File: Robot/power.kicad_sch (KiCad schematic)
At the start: 34 parts, among them J16 Battery, J17 DE9_Receptacle, J18 Balance, Q1 DMP3036SSD, Q2 Si2003, SW2 Pwr, U4 ICE40UP5K-SG48ITR, U7 NC7SZ175, U8 TLV70212DBVR, U9 TMI6050-33

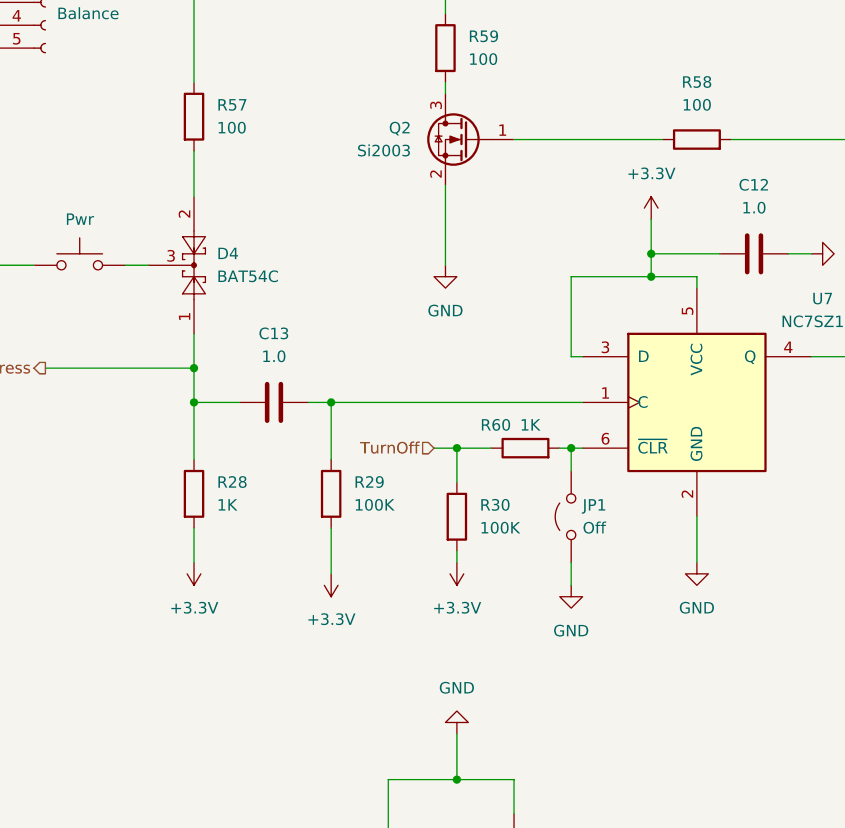
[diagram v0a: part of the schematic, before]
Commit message: Updated PCB for Robot (routing in progress)
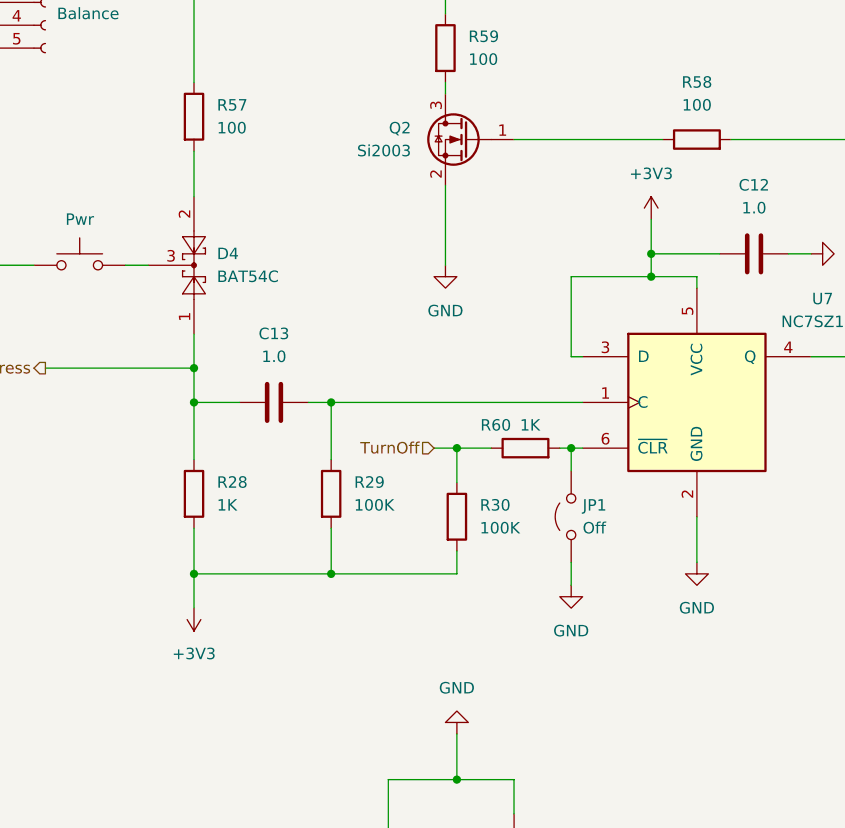
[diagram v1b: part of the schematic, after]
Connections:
- net +3.3V is gone; now on net +3V3: C12.1, R28.2, R29.2, R30.2, U7.3 (D), U7.5 (VCC)
